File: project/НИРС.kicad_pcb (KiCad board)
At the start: 2 copper layers, 58.9 x 53.3 mm, 79 parts, among them J10 J10, J7 J7, J8 J8, J9 J9, Q301 Tran_8050, Q302 Tran_8050, Q303 Tran_8050, Q304 Tran_8050, Q305 Tran_8050, Q306 Tran_8050, Q307 Tran_8050, Q308 Tran_8050, U201 74HC595, U202 74HC595, j6 J6

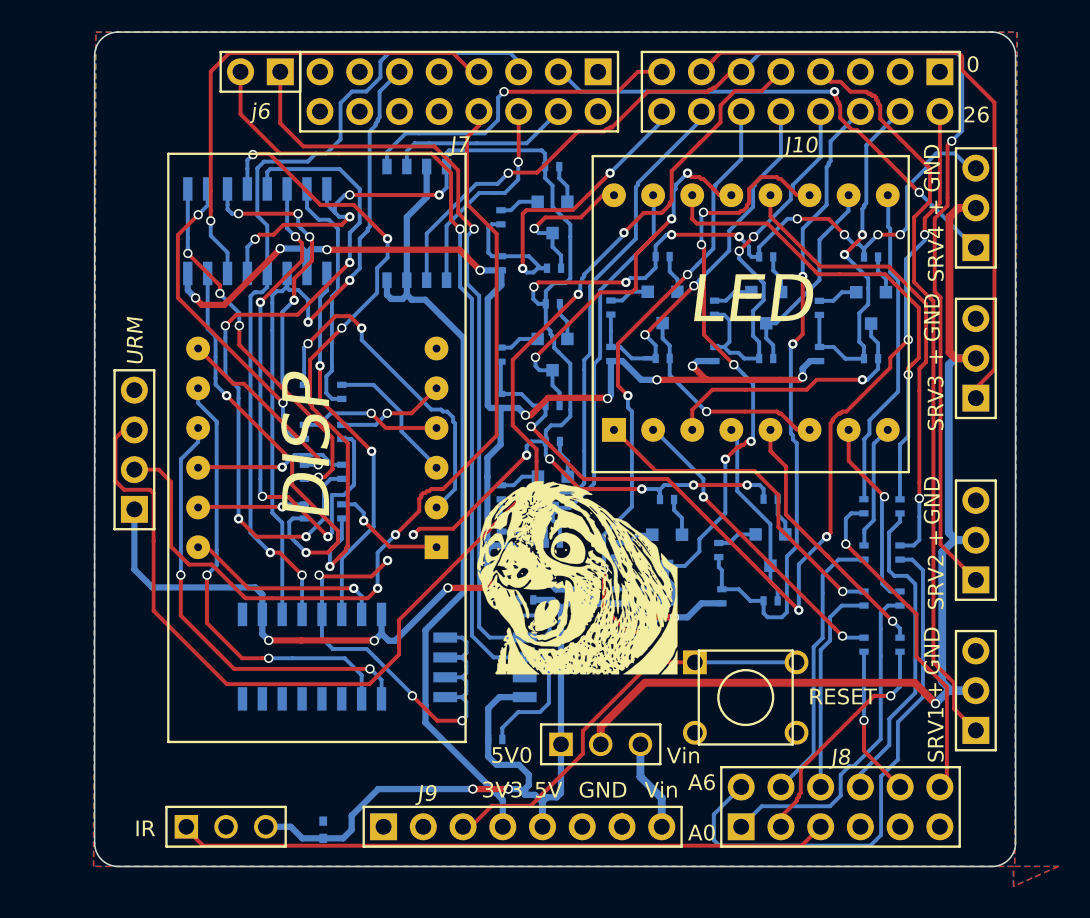
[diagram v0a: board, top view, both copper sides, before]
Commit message: Add files via upload
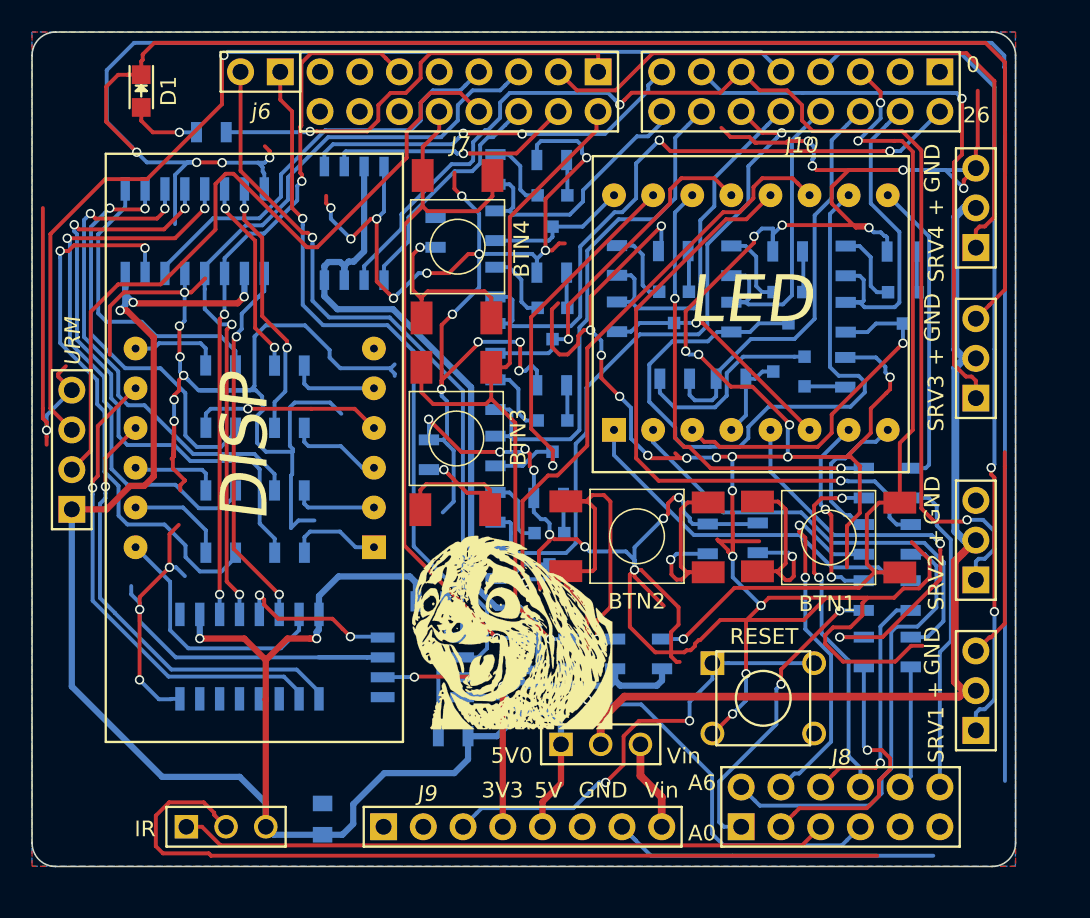
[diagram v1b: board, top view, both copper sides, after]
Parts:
- removed R101, R102, R103, R104, R105, R106, R107, R108: 4,7K, Resistors_SMD:R_0402
- added BTN1: Button, WIFIRE:BUTTON, F.Cu at (182.1, 128.8)
- added BTN2: Button, WIFIRE:BUTTON, F.Cu at (169.9, 128.8)
- added BTN3: Button, WIFIRE:BUTTON, F.Cu at (158.3, 122.5)
- added BTN4: Button, WIFIRE:BUTTON, F.Cu at (158.4, 110.2)
- added D1: LED, LEDs:LED_0805, F.Cu at (138.2, 100.3)
- added R111: 220, Resistors_SMD:R_0805, B.Cu at (142.7, 102.9)
- added R112: 10K, Resistors_SMD:R_0805, B.Cu at (171.5, 136.3)
- added R113: 10K, Resistors_SMD:R_0805, B.Cu at (168.5, 136.3)
- added R114: 220, Resistors_SMD:R_0805, B.Cu at (177.6, 128.8)
- added R115: 220, Resistors_SMD:R_0805, B.Cu at (174.4, 128.9)
- added R116: 10K, Resistors_SMD:R_0805, B.Cu at (165.5, 136.3)
- added R117: 10K, Resistors_SMD:R_0805, B.Cu at (162.5, 136.3)
- added R118: 220, Resistors_SMD:R_0805, B.Cu at (156.6, 123.5)
- added R119: 220, Resistors_SMD:R_0805, B.Cu at (157.0, 109.3)
- C101: footprint Capacitors_SMD:C_0402 -> Capacitors_SMD:C_0805
- R109, R110, R201, R202, R203, R204, R205, R206, R207, R208, R301, R302, R303, R304, R305, R306, R307, R308, R309, R310, R311, R312, R313, R314, R315, R316, R317, R318, R319, R320, R321, R322, R323, R324, R325, R326, R327, R328, R329, R330, R331, R332: footprint Resistors_SMD:R_0402 -> Resistors_SMD:R_0805
- moved R323 14.4 mm to (175.9, 118.7)
- moved Q306 11.5 mm to (179.6, 118.2), turned to 270 degrees
- moved R324 11.3 mm to (172.3, 118.7), turned to 0 degrees
- moved R321 11.2 mm to (160.8, 130.5), turned to 270 degrees
- moved R326 9.41 mm to (183.2, 118.3), turned to 270 degrees
- moved R202 8.66 mm to (143.2, 117.8), turned to 180 degrees
- moved R322 8.15 mm to (160.8, 126.9)
- moved R206 7.83 mm to (143.3, 125.8), turned to 180 degrees
- moved R325 7.57 mm to (164.2, 126.3)
- moved Q305 7.53 mm to (164.3, 129.6)
- moved R315 6.94 mm to (160.8, 123.3), turned to 270 degrees
- moved R204 6.37 mm to (147.7, 125.8), turned to 0 degrees
- moved R316 6.25 mm to (160.8, 119.7)
- moved R109 6.10 mm to (156.7, 132.9), turned to 180 degrees
- moved R201 5.97 mm to (143.3, 129.8), turned to 180 degrees
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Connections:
- J10 pad 5: Net-(J10-Pad5) -> /BTN_1
- J7 pad 10: Net-(J7-Pad10) -> /BTN_4
- J7 pad 2: Net-(J7-Pad2) -> /BTN_3
- J8 pad 7: Net-(J8-Pad7) -> /BTN_2
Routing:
- net GND: track 156.7 -> 776.8 mm, vias 22 -> 66
- net /BTN_1: track 0.00 -> 55.4 mm, vias 0 -> 3
- net /BTN_2: track 0.00 -> 54.3 mm, vias 0 -> 2
- net +5V: track 180.7 -> 127.6 mm, vias 17 -> 5
- net /BTN_3: track 0.00 -> 46.3 mm, vias 0 -> 1
- net /BTN_4: track 0.00 -> 44.9 mm, vias 0 -> 1
- net /LED/GNM_10: track 13.4 -> 44.4 mm
- net Net-(J7-Pad1): track 0.00 -> 28.2 mm, vias 0 -> 1
- net /LED/COL1: track 65.2 -> 41.4 mm, vias 5 -> 2
- net Net-(R207-Pad1): track 34.6 -> 12.6 mm, vias 4 -> 2
- net +3V3: track 50.4 -> 69.6 mm, vias 0 -> 1
- net /7-SEGM/QD: track 22.3 -> 5.40 mm, vias 2 -> 0
- net /Echo: track 83.2 -> 66.9 mm, vias 2 -> 1
- net /LED/COL3: track 42.2 -> 26.6 mm, vias 2 -> 0
- net Net-(BTN1-Pad3): track 0.00 -> 12.5 mm, vias 0 -> 1
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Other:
- board size 58.9 x 53.3 mm -> 62.9 x 53.3 mm
- board text added: "4,7K"
- board text added: "68"
- board text removed: "4k7"
